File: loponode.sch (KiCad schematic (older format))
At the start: 20 parts

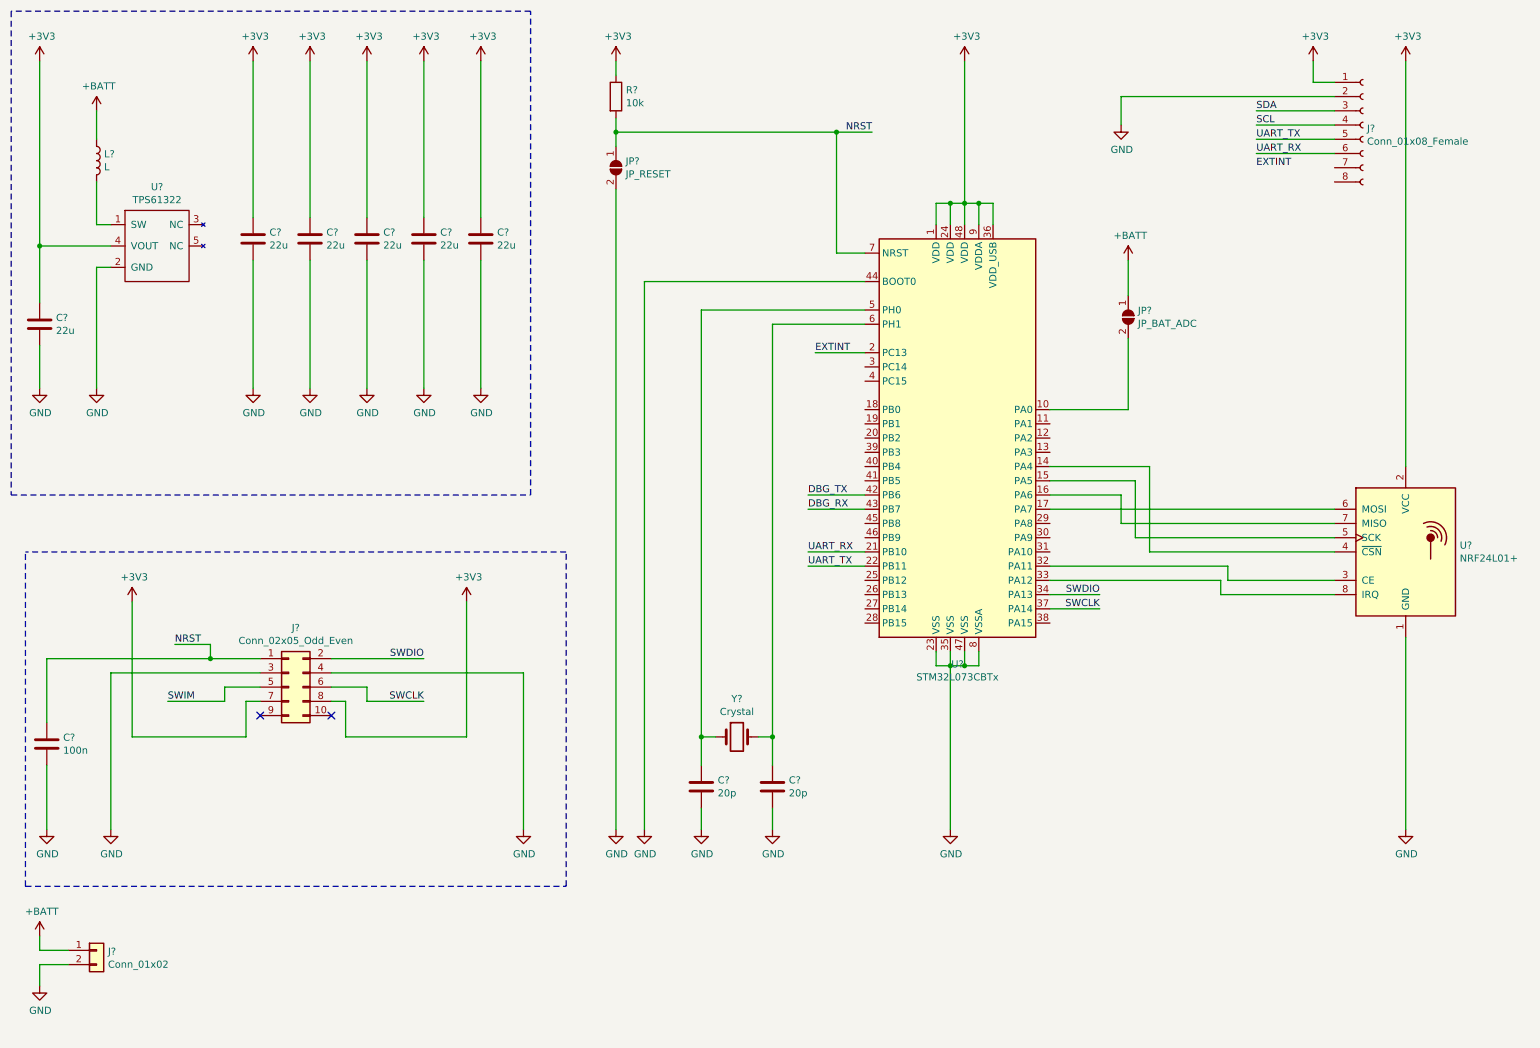
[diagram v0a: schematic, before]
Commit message: some fixes, annotations, associations
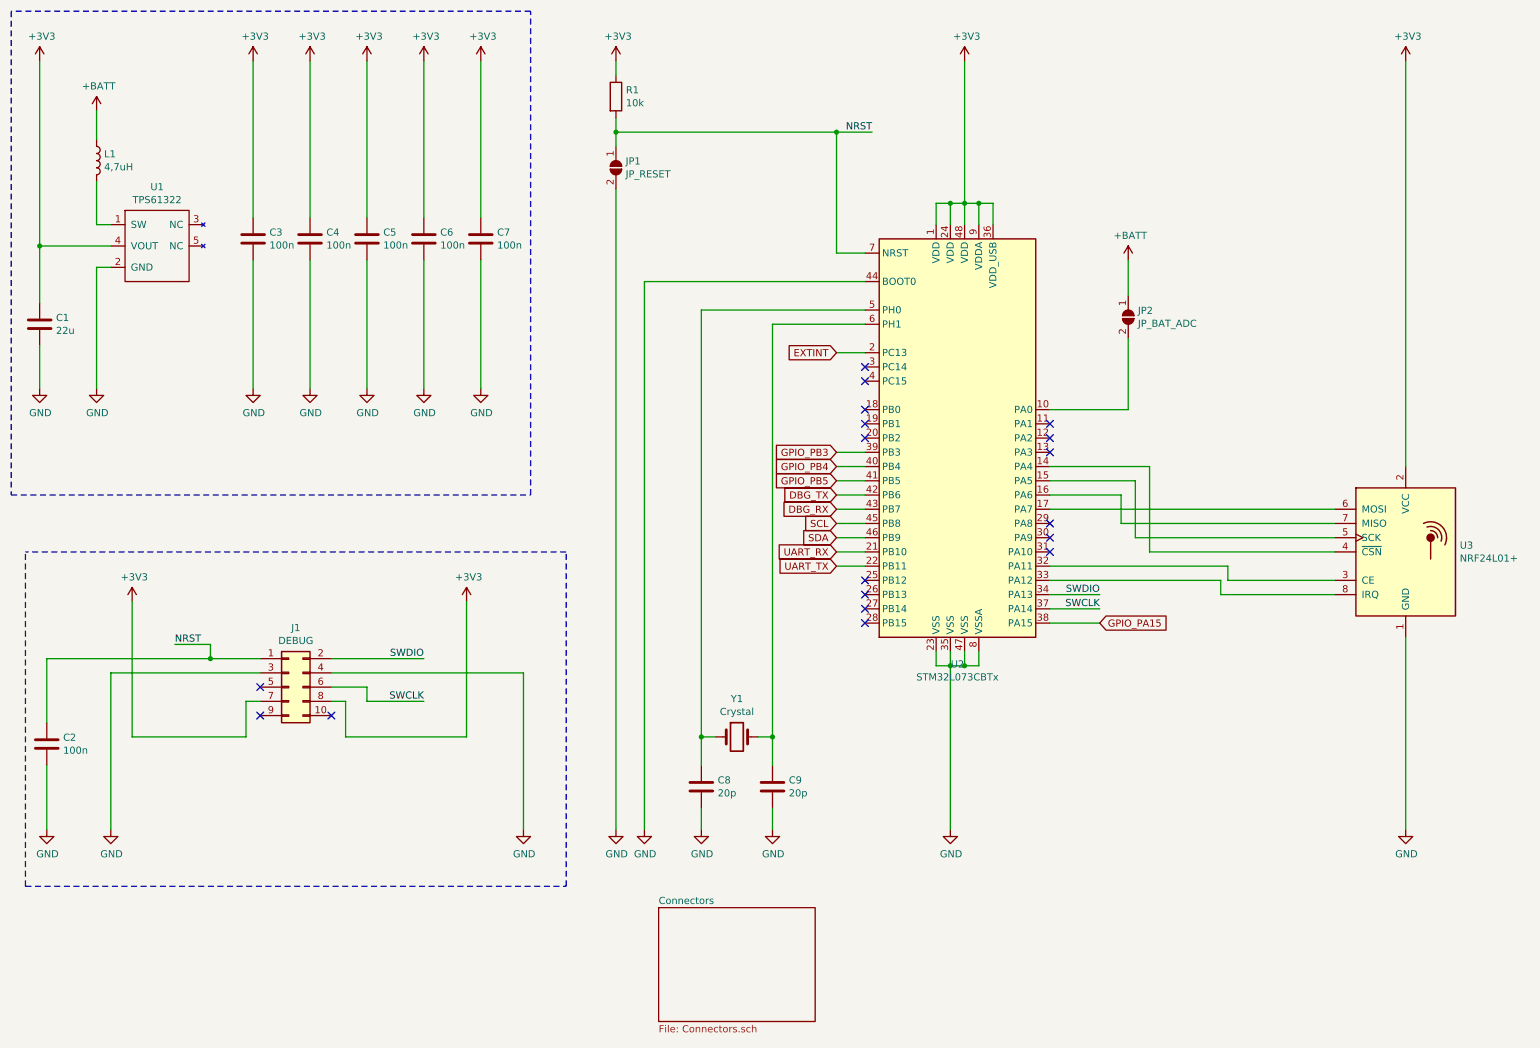
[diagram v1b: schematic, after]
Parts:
- removed J?: Conn_01x08_Female, symbol Connector:Conn_01x08_Female
- removed J?: Conn_01x02, symbol Connector_Generic:Conn_01x02
- C1, C2, C8, C9: renamed from C?; footprint (none) -> Capacitor_SMD:C_0805_2012Metric_Pad1.15x1.40mm_HandSolder
- C3, C4, C5, C6, C7: renamed from C?; value 22u -> 100n; footprint (none) -> Capacitor_SMD:C_0805_2012Metric_Pad1.15x1.40mm_HandSolder
- J1: renamed from J?; value Conn_02x05_Odd_Even -> DEBUG; footprint (none) -> Connector_PinHeader_2.54mm:PinHeader_2x05_P2.54mm_Vertical
- JP1, JP2: renamed from JP?; footprint (none) -> Jumper:SolderJumper-2_P1.3mm_Open_TrianglePad1.0x1.5mm
- L1: renamed from L?; value L -> 4,7uH
- R1: renamed from R?; footprint (none) -> Resistor_SMD:R_0805_2012Metric_Pad1.15x1.40mm_HandSolder
- gave numbers to parts that had none: 4
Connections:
- net SCL: now also U2.45 (PB8)
- net SDA: now also U2.46 (PB9)
- net GPIO_PA15: now reaches U2.38 (PA15)
- net GPIO_PB3: now reaches U2.39 (PB3)
- net GPIO_PB4: now reaches U2.40 (PB4)
- net GPIO_PB5: now reaches U2.41 (PB5)
- net SWIM: no longer names the net of J1.5 (Pin_5)
- no-connect marks 2 -> 18
